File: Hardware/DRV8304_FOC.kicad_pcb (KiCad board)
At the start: 4 copper layers, 55 x 55 mm, 74 parts, among them J1 Conn_01x02, J3 Conn_01x03, J4 Conn_02x07_Counter_Clockwise, Q1 SIRA18ADP, Q2 SIRA18ADP, Q3 SIRA18ADP, Q4 SIRA18ADP, Q5 SIRA18ADP, Q6 SIRA18ADP, SW2 SW_Push, U1 TPS565208, U2 TPS259850RQPR, U3 DRV8304HRHAR, U4 STM32F412CEUx, U5 AS5055A, Y1 Crystal_GND23

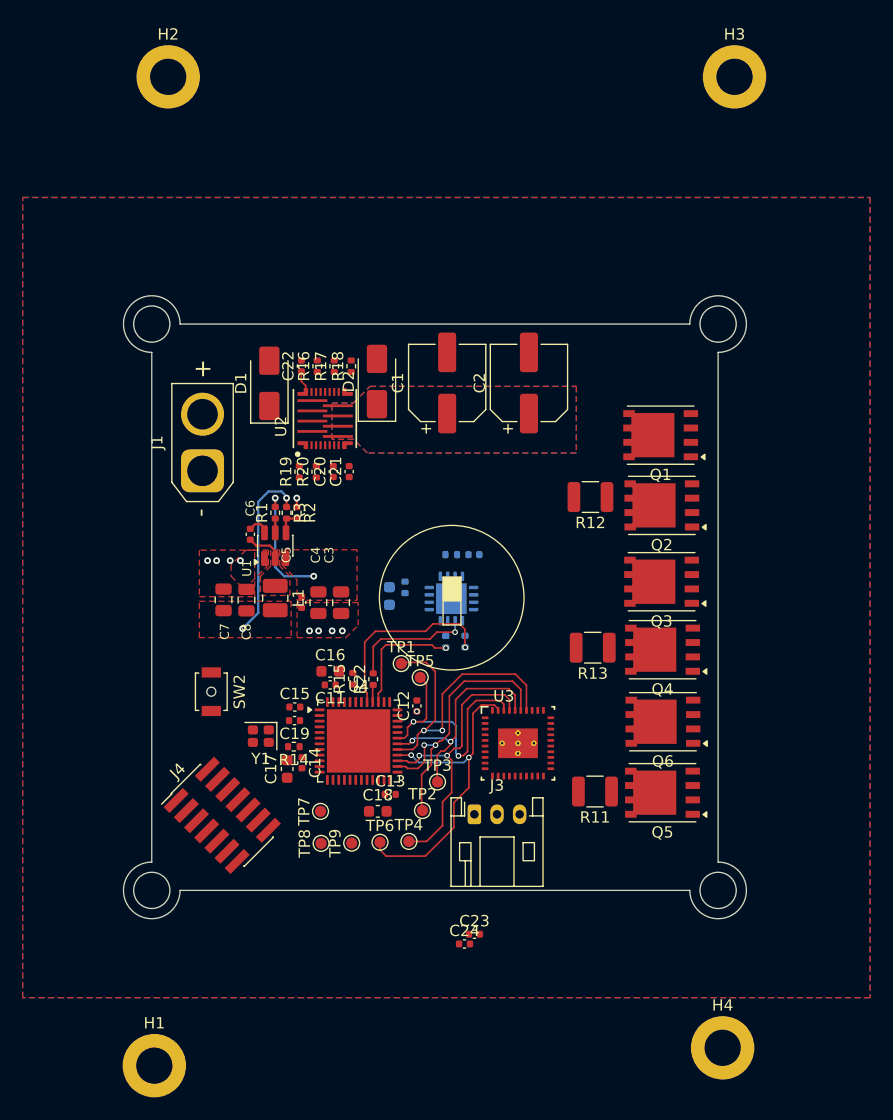
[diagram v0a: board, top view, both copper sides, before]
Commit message: Routing update
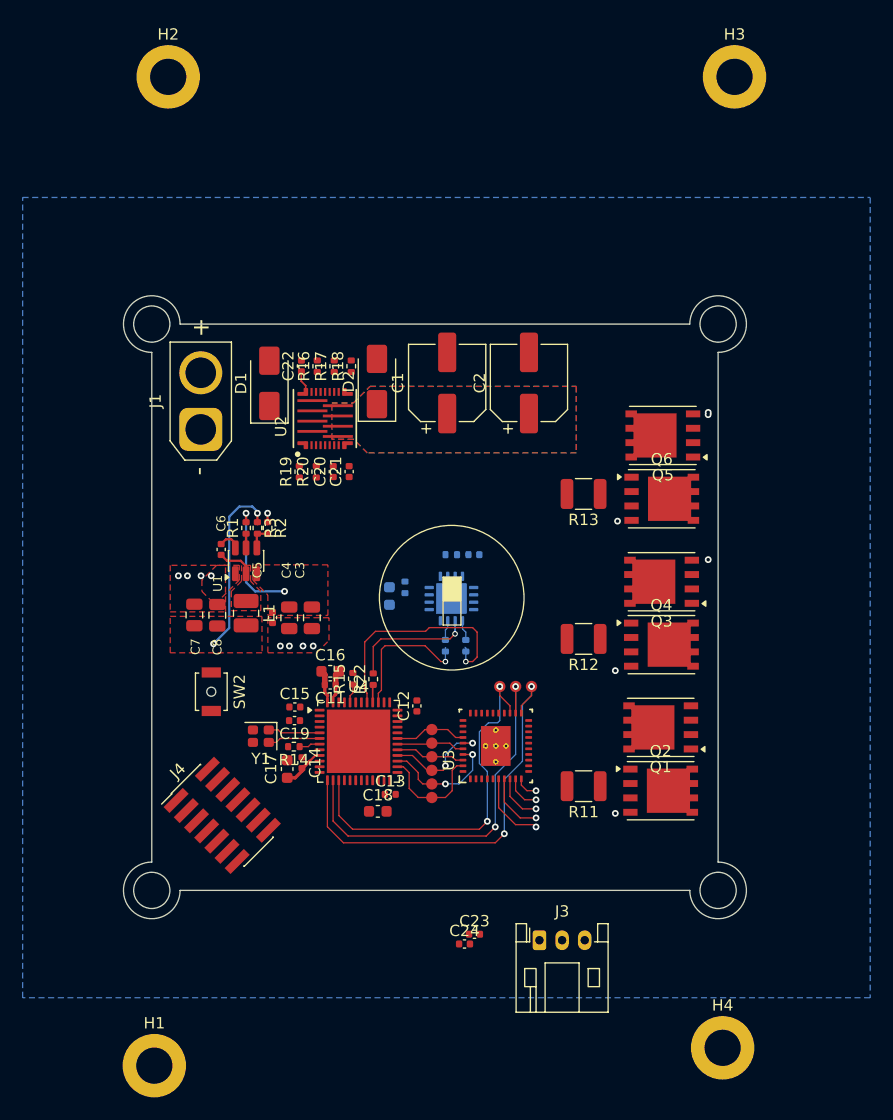
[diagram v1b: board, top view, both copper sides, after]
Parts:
- TP1, TP2, TP3, TP4, TP5, TP6, TP7, TP8, TP9: footprint TestPoint:TestPoint_Pad_D1.0mm -> MyLib:TestPoint_1mm
- moved Q5 31.5 mm to (180.7, 82.4)
- moved Q1 25.8 mm to (180.5, 108.2)
- moved Q2 25.2 mm to (180.5, 113.8), turned to 0 degrees
- moved TP8 22.1 mm to (167.7, 104.6)
- moved TP7 21.6 mm to (169.1, 104.6)
- moved Q6 19.7 mm to (180.6, 88.0), turned to 0 degrees
- moved TP9 19.0 mm to (166.3, 104.6)
- moved R13 13.6 mm to (173.7, 87.6)
- moved R12 12.5 mm to (173.7, 100.4)
- moved J3 12.5 mm to (169.8, 127.0)
- moved TP5 7.07 mm to (160.3, 110.8)
- moved TP1 6.42 mm to (160.3, 108.4)
- moved TP6 6.04 mm to (160.3, 114.4)
- moved TP4 5.46 mm to (160.3, 113.2)
- moved J1 3.66 mm to (139.9, 81.9)
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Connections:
- Q1 pad 1: Net-(Q1-D) -> SHA
- Q1 pad 2: Net-(Q1-D) -> SHA
- Q1 pad 3: Net-(Q1-D) -> SHA
- Q2 pad 5: Net-(Q1-D) -> SHA
- Q3 pad 1: Net-(Q3-D) -> SHB
- Q3 pad 2: Net-(Q3-D) -> SHB
- Q3 pad 3: Net-(Q3-D) -> SHB
- Q3 pad 4: unconnected-(Q3-G-Pad4) -> GHB
- Q4 pad 4: unconnected-(Q4-G-Pad4) -> GLB
- Q4 pad 5: Net-(Q3-D) -> SHB
- Q5 pad 1: Net-(Q5-D) -> SHC
- Q5 pad 2: Net-(Q5-D) -> SHC
- Q5 pad 3: Net-(Q5-D) -> SHC
- Q5 pad 4: unconnected-(Q5-G-Pad4) -> GHC
- Q6 pad 4: unconnected-(Q6-G-Pad4) -> GLC
- Q6 pad 5: Net-(Q5-D) -> SHC
- U4 pad 26: INLA -> INLC
- U4 pad 28: INLC -> INLA
- U4 pad 29: INHA -> INHC
- U4 pad 31: INHC -> INHA
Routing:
- net ISENSE_C: track 0.00 -> 37.6 mm, vias 0 -> 2
- net ISENSE_B: track 0.00 -> 34.3 mm, vias 0 -> 2
- net ISENSE_A: track 0.00 -> 33.1 mm, vias 0 -> 2
- net INHA: track 28.6 -> 6.40 mm, vias 2 -> 0
- net INLC: track 28.8 -> 9.94 mm, vias 2 -> 0
- net INHC: track 23.1 -> 6.16 mm, vias 2 -> 0
- net INLA: track 25.5 -> 9.72 mm
- net INLB: track 26.1 -> 10.6 mm
- net INHB: track 20.7 -> 6.03 mm, vias 2 -> 0
- net 3V3: track 0.00 -> 6.80 mm
- net GHA: track 0.00 -> 6.55 mm, vias 0 -> 1
- net SHA: track 0.00 -> 5.43 mm, vias 0 -> 1
- net Net-(U4-PH1): track 0.00 -> 4.63 mm
- net Net-(U4-PH0): track 0.00 -> 4.59 mm
- net GLA: track 0.00 -> 4.31 mm, vias 0 -> 1
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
